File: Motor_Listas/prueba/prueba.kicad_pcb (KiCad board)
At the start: 2 copper layers, 40 x 25 mm, 2 parts

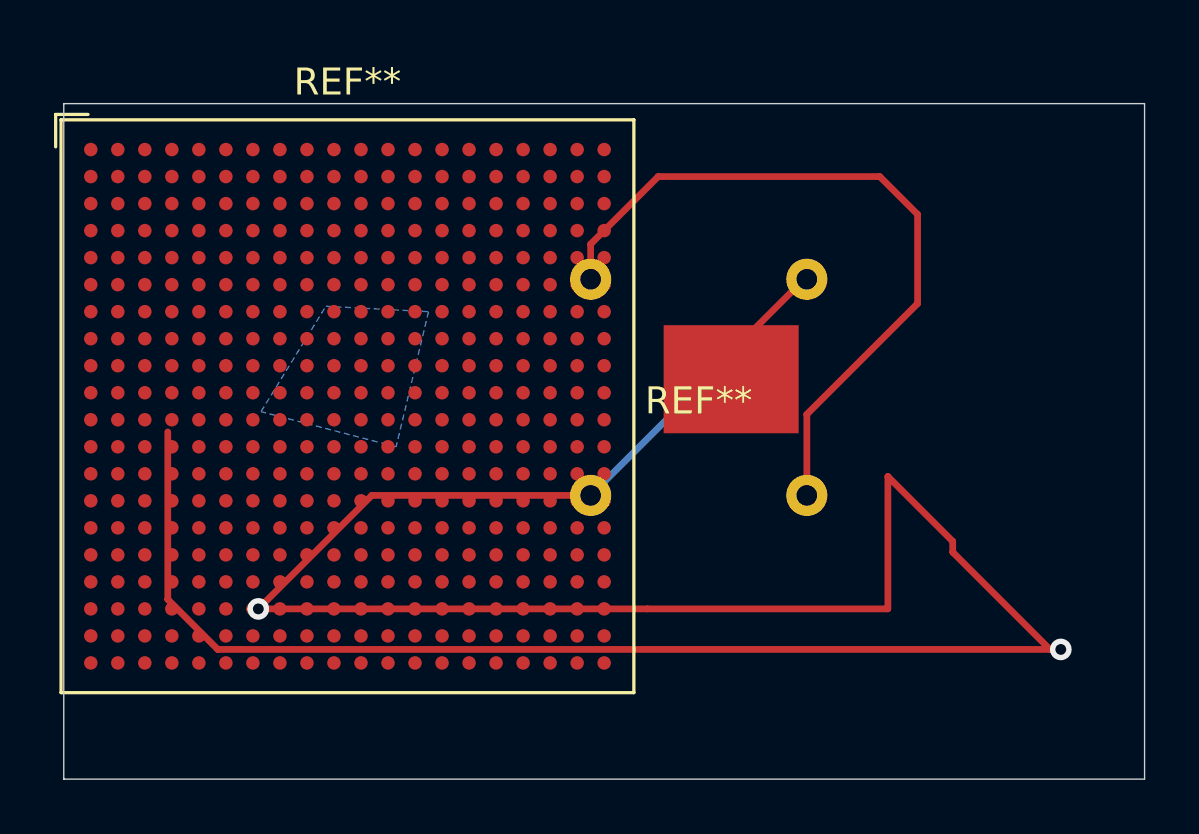
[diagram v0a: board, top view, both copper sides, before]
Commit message: update
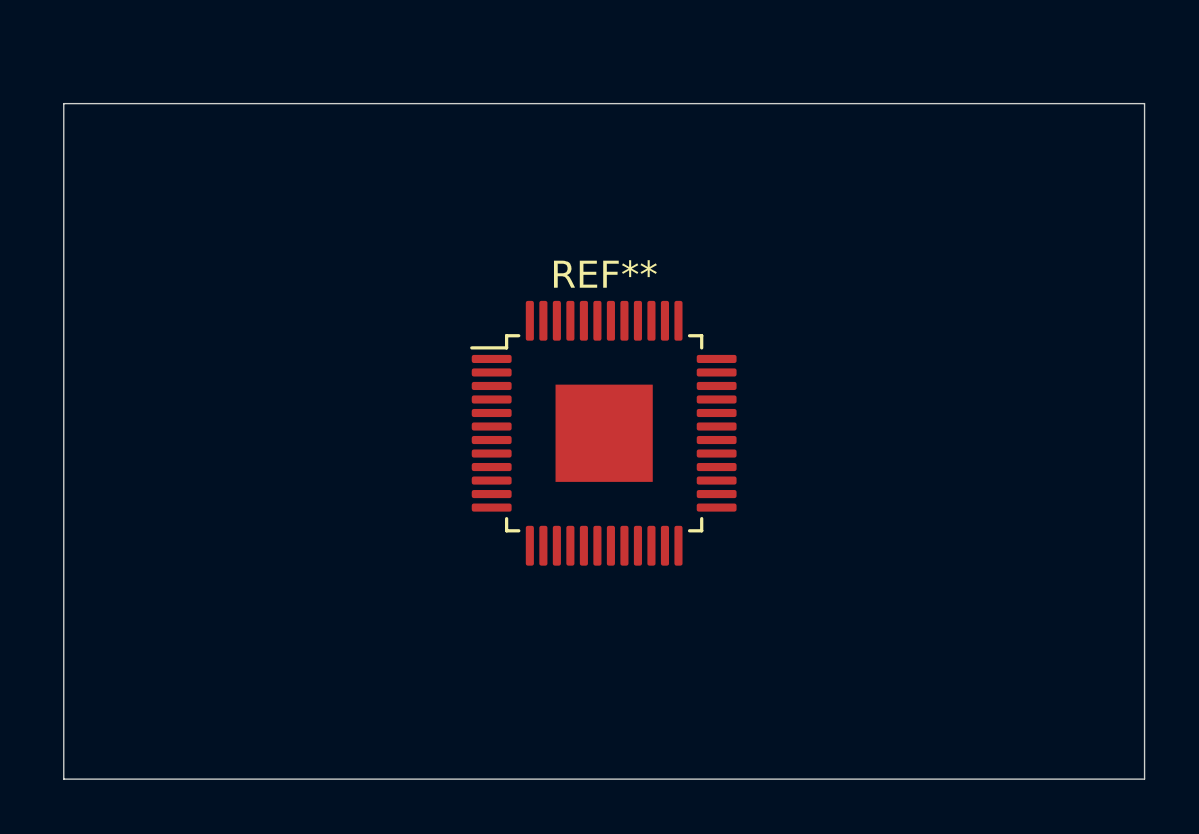
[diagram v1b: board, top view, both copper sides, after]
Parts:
- removed the REF** at (113.5, 25.5)
- removed the REF** at (100.5, 26.2)
- added REF**: LQFP-48-1EP_7x7mm_P0.5mm_EP3.6x3.6mm, Package_QFP:LQFP-48-1EP_7x7mm_P0.5mm_EP3.6x3.6mm, F.Cu at (110.0, 27.2)
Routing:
- net (no net): track 130.0 -> 0.00 mm, vias 2 -> 0
- removed copper zone on B.Cu, net (none)
